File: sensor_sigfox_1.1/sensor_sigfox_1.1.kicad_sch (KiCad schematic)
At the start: 18 parts, among them IC1 WSSFM11R2DAT, J1 Battery, J2 Conn_01x07_Socket, J3 Conn_01x01_Female, J4 Antenna, U1 ATtiny826-X, U2 MLX90393, Y1 32.768 kHz

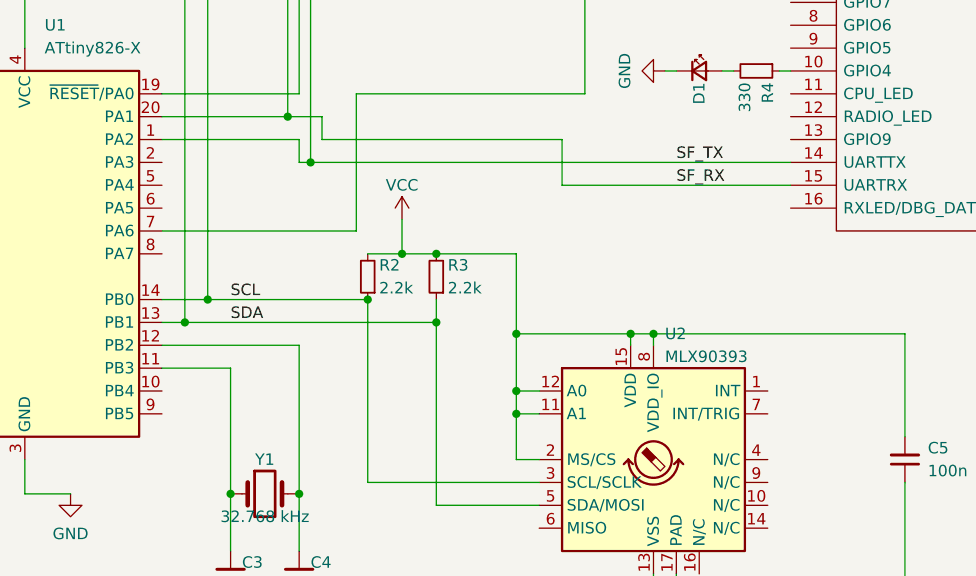
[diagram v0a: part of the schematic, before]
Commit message: gerber y conexiones int/trig
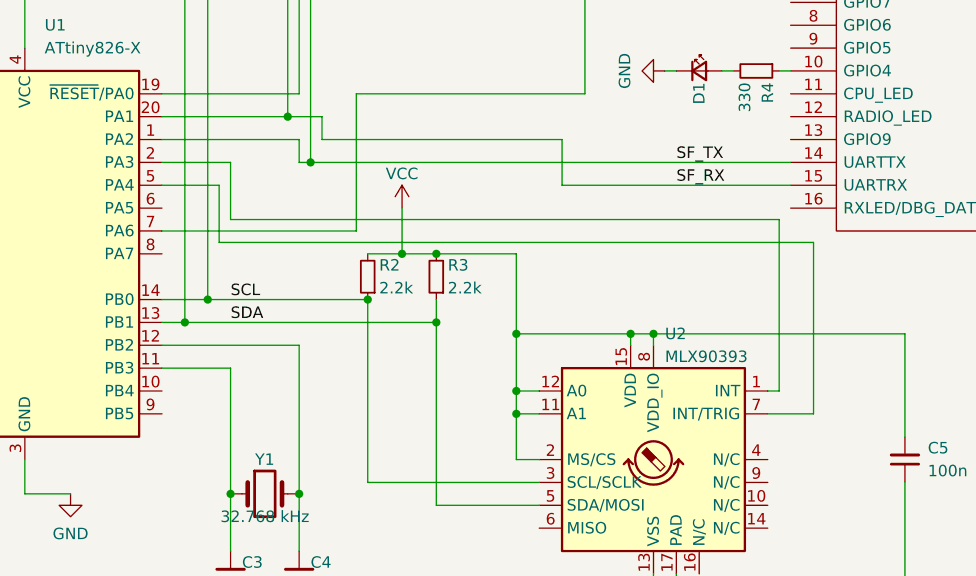
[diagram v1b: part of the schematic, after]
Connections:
- net at U1.2 (PA3): now also U2.1 (INT)
- net at U1.5 (PA4): now also U2.7 (INT/TRIG)
